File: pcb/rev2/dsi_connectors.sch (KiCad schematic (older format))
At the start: 6 parts, among them CN2 AX3E41264, CN3 CONN_02X15_ALT

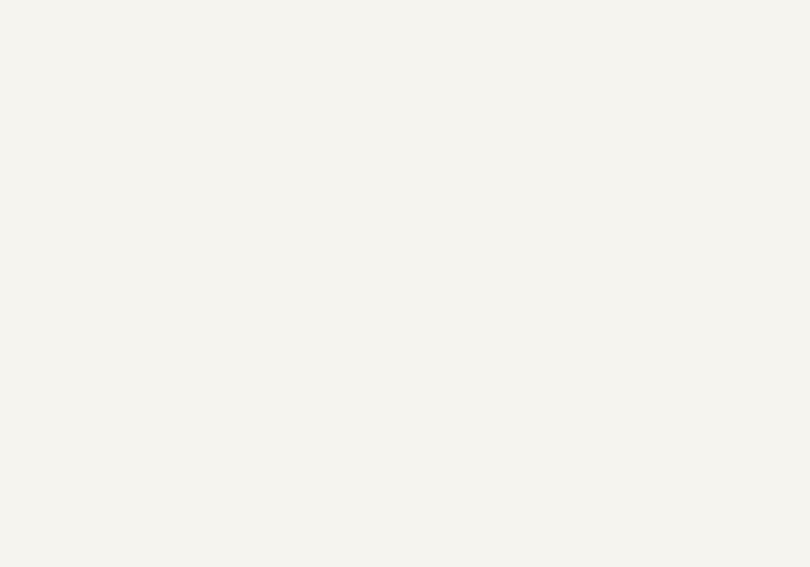
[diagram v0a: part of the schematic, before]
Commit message: pcb wip
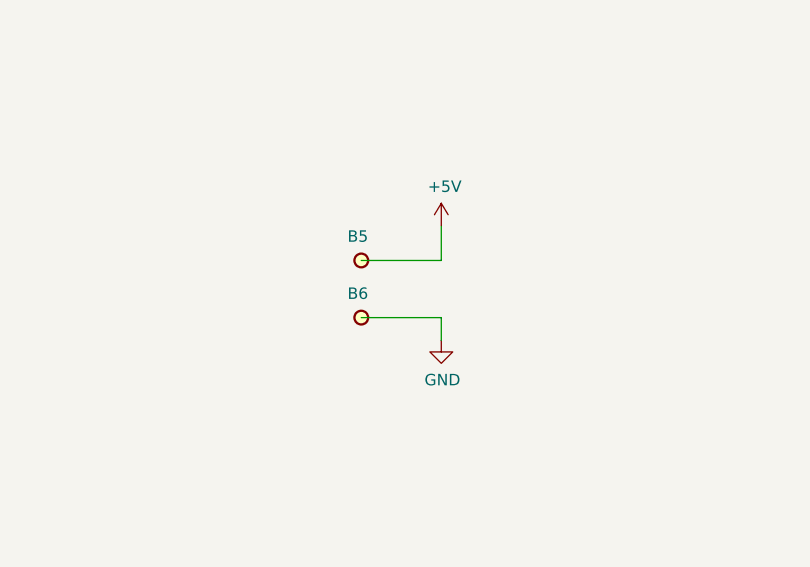
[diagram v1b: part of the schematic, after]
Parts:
- added B5, B6: PLATED_HOLE0.8_PAD1.3, c130h80, symbol PLATED_HOLE0.8_PAD1.3
- CN2: footprint (none) -> dsi_shield:IPHONE4_LCD_CONN
- CN3: footprint (none) -> dsi_shield:GB042-30S-E1000
- R1, R2, R49, R50: footprint RESC1608X55N -> Resistors SMD:RESC1608X55N
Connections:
- net labels added: +5V
- wire segments 79 -> 83
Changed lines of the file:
@@
 F 0 "CN2" H 6450 2865 50  0000 C CNN
 F 1 "AX3E41264" H 6450 2774 50  0000 C CNN
-F 2 "" H 6450 900 50  0001 C CNN
+F 2 "dsi_shield:IPHONE4_LCD_CONN" H 6450 900 50  0001 C CNN
 F 3 "" H 6450 900 50  0001 C CNN
 	1    6450 2050
@@
 F 0 "R1" H 7650 1853 50  0000 C CNN
 F 1 "R0603_10R_1%_0.1W_200PPM" H 7500 1340 60  0001 L CNN
-F 2 "RESC1608X55N" H 7500 530 60  0001 L CNN
+F 2 "Resistors SMD:RESC1608X55N" H 7500 530 60  0001 L CNN
 F 3 "\\cern.ch\\dfs\\Applications\\Altium\\Datasheets\\R0603_NIC_NRC.pdf" H 7500 1160 60  0001 L CNN
 F 4 "Value" H 7500 1550 60  0001 C CNN "Fieldname"
@@
 F 0 "R2" H 7650 2147 50  0000 C CNN
 F 1 "R0603_3K3_1%_0.1W_100PPM" H 7500 1740 60  0001 L CNN
-F 2 "RESC1608X55N" H 7500 930 60  0001 L CNN
+F 2 "Resistors SMD:RESC1608X55N" H 7500 930 60  0001 L CNN
 F 3 "\\cern.ch\\dfs\\Applications\\Altium\\Datasheets\\R0603_NIC_NRC.pdf" H 7500 1560 60  0001 L CNN
 F 4 "3k3" H 7650 2056 50  0000 C CNN "~"
@@
 F 0 "CN3" H 6450 5865 50  0000 C CNN
 F 1 "CONN_02X15_ALT" H 6450 5774 50  0000 C CNN
-F 2 "" H 6450 3800 50  0001 C CNN
+F 2 "dsi_shield:GB042-30S-E1000" H 6450 3800 50  0001 C CNN
 F 3 "" H 6450 3800 50  0001 C CNN
 	1    6450 4950
@@
 F 0 "R49" H 7300 4547 50  0000 C CNN
 F 1 "R0603_10R_1%_0.1W_200PPM" H 7150 4140 60  0001 L CNN
-F 2 "RESC1608X55N" H 7150 3330 60  0001 L CNN
+F 2 "Resistors SMD:RESC1608X55N" H 7150 3330 60  0001 L CNN
 F 3 "\\cern.ch\\dfs\\Applications\\Altium\\Datasheets\\R0603_NIC_NRC.pdf" H 7150 3960 60  0001 L CNN
 F 4 "10" H 7300 4456 50  0000 C CNN "~"
@@
 F 0 "R50" H 7300 4345 50  0000 C CNN
 F 1 "R0603_10R_1%_0.1W_200PPM" H 7150 4240 60  0001 L CNN
-F 2 "RESC1608X55N" H 7150 3430 60  0001 L CNN
+F 2 "Resistors SMD:RESC1608X55N" H 7150 3430 60  0001 L CNN
 F 3 "\\cern.ch\\dfs\\Applications\\Altium\\Datasheets\\R0603_NIC_NRC.pdf" H 7150 4060 60  0001 L CNN
 F 4 "10" H 7450 4350 50  0000 C CNN "~"
@@
 Wire Notes Line
 	3100 6800 700  6800
+$Comp
+L PLATED_HOLE0.8_PAD1.3 B5
+U 1 1 599E1A70
+P 2500 5000
+F 0 "B5" H 2485 5105 50  0000 C CNN
+F 1 "PLATED_HOLE0.8_PAD1.3" H 2500 4830 60  0001 L CNN
+F 2 "c130h80" H 2500 4020 60  0001 L CNN
+F 3 "Undefined" H 2500 4650 60  0001 L CNN
+F 4 "Plated Hole" H 2500 4560 60  0001 L CNN "Field4"
+F 5 "PLATED_HOLE0.8_PAD1.3" H 2500 4560 60  0001 L CNN "Part Number"
+F 6 "Single Terminal Socket" H 2500 4470 60  0001 L CNN "Library Ref"
+F 7 "SchLib\\Pads.SchLib" H 2500 4380 60  0001 L CNN "Library Path"
+F 8 "~~" H 2500 4290 60  0001 L CNN "Comment"
+F 9 "Standard (No BOM)" H 2500 4200 60  0001 L CNN "Component Kind"
+F 10 "Standard (No BOM)" H 2500 4110 60  0001 L CNN "Component Type"
+F 11 "1" H 2500 3930 60  0001 L CNN "Pin Count"
+F 12 "~~" H 2500 3840 60  0001 L CNN "Case"
+F 13 "PcbLib\\Pads.PcbLib" H 2500 3750 60  0001 L CNN "Footprint Path"
+F 14 "c130h80" H 2500 3660 60  0001 L CNN "Footprint Ref"
+F 15 "Plated Hole" H 2500 3570 60  0001 L CNN "Family"
+F 16 "No" H 2500 3480 60  0001 L CNN "Mounted"
+F 17 "No" H 2500 3390 60  0001 L CNN "Socket"
+F 18 "No" H 2500 3300 60  0001 L CNN "SMD"
+F 19 "No" H 2500 3210 60  0001 L CNN "Sense"
+F 20 "~~" H 2500 3120 60  0001 L CNN "Sense Comment"
+F 21 "None" H 2500 3030 60  0001 L CNN "Status"
+F 22 "~~" H 2500 2940 60  0001 L CNN "Status Comment"
+F 23 "~~" H 2500 2850 60  0001 L CNN "SCEM"
+F 24 "Plated Through Hole: Hole Dia.=0.8mm Pad Dia.=1.3mm, IPC-7251 Level C" H 2500 2760 60  0001 L CNN "Part Description"
+F 25 "~~" H 2500 2670 60  0001 L CNN "Manufacturer"
+F 26 "~~" H 2500 2580 60  0001 L CNN "Manufacturer Part Number"
+F 27 "0mm" H 2500 2490 60  0001 L CNN "ComponentHeight"
+F 28 "~~" H 2500 2400 60  0001 L CNN "Manufacturer1 Example"
+F 29 "~~" H 2500 2310 60  0001 L CNN "Manufacturer1 Part Number"
+F 30 "~~" H 2500 2220 60  0001 L CNN "Manufacturer1 ComponentHeight"
+F 31 "Undefined" H 2500 2130 60  0001 L CNN "HelpURL"
+F 32 "~~" H 2500 2040 60  0001 L CNN "ComponentLink1URL"
+F 33 "~~" H 2500 1950 60  0001 L CNN "ComponentLink1Description"
+F 34 "~~" H 2500 1860 60  0001 L CNN "ComponentLink2URL"
+F 35 "~~" H 2500 1770 60  0001 L CNN "ComponentLink2Description"
+F 36 "CERN DEM JLC" H 2500 1680 60  0001 L CNN "Author"
+F 37 "10/30/08 00:00:00" H 2500 1590 60  0001 L CNN "CreateDate"
+F 38 "10/30/08 00:00:00" H 2500 1500 60  0001 L CNN "LatestRevisionDate"
+F 39 "Plated Through Hole: Hole Dia.=0.8mm Pad Dia.=1.3mm, IPC-7251 Level C" H 2500 1410 60  0001 L CNN "PackageDescription"
+F 40 "Pads" H 2500 1320 60  0001 L CNN "Library Name"
+F 41 "This work is licensed under the Creative Commons CC-BY-SA 4.0 License. To the extent that circuit schematics that use Licensed Material can be considered to be ‘Adapted Material’, then the copyright holder waives article 3.b of the license with respect to these schematics." H 2500 1230 60  0001 L CNN "License"
+	1    2500 5000
+	1    0    0    -1
+$EndComp
+$Comp
+L PLATED_HOLE0.8_PAD1.3 B6
+U 1 1 599E1C02
+P 2500 5250
+F 0 "B6" H 2485 5355 50  0000 C CNN
+F 1 "PLATED_HOLE0.8_PAD1.3" H 2500 5080 60  0001 L CNN
+F 2 "c130h80" H 2500 4270 60  0001 L CNN
+F 3 "Undefined" H 2500 4900 60  0001 L CNN
+F 4 "Plated Hole" H 2500 4810 60  0001 L CNN "Field4"
+F 5 "PLATED_HOLE0.8_PAD1.3" H 2500 4810 60  0001 L CNN "Part Number"
+F 6 "Single Terminal Socket" H 2500 4720 60  0001 L CNN "Library Ref"
+F 7 "SchLib\\Pads.SchLib" H 2500 4630 60  0001 L CNN "Library Path"
+F 8 "~~" H 2500 4540 60  0001 L CNN "Comment"
+F 9 "Standard (No BOM)" H 2500 4450 60  0001 L CNN "Component Kind"
+F 10 "Standard (No BOM)" H 2500 4360 60  0001 L CNN "Component Type"
+F 11 "1" H 2500 4180 60  0001 L CNN "Pin Count"
+F 12 "~~" H 2500 4090 60  0001 L CNN "Case"
+F 13 "PcbLib\\Pads.PcbLib" H 2500 4000 60  0001 L CNN "Footprint Path"
+F 14 "c130h80" H 2500 3910 60  0001 L CNN "Footprint Ref"
+F 15 "Plated Hole" H 2500 3820 60  0001 L CNN "Family"
+F 16 "No" H 2500 3730 60  0001 L CNN "Mounted"
+F 17 "No" H 2500 3640 60  0001 L CNN "Socket"
+F 18 "No" H 2500 3550 60  0001 L CNN "SMD"
+F 19 "No" H 2500 3460 60  0001 L CNN "Sense"
+F 20 "~~" H 2500 3370 60  0001 L CNN "Sense Comment"
+F 21 "None" H 2500 3280 60  0001 L CNN "Status"
+F 22 "~~" H 2500 3190 60  0001 L CNN "Status Comment"
+F 23 "~~" H 2500 3100 60  0001 L CNN "SCEM"
+F 24 "Plated Through Hole: Hole Dia.=0.8mm Pad Dia.=1.3mm, IPC-7251 Level C" H 2500 3010 60  0001 L CNN "Part Description"
+F 25 "~~" H 2500 2920 60  0001 L CNN "Manufacturer"
+F 26 "~~" H 2500 2830 60  0001 L CNN "Manufacturer Part Number"
+F 27 "0mm" H 2500 2740 60  0001 L CNN "ComponentHeight"
+F 28 "~~" H 2500 2650 60  0001 L CNN "Manufacturer1 Example"
+F 29 "~~" H 2500 2560 60  0001 L CNN "Manufacturer1 Part Number"
+F 30 "~~" H 2500 2470 60  0001 L CNN "Manufacturer1 ComponentHeight"
+F 31 "Undefined" H 2500 2380 60  0001 L CNN "HelpURL"
+F 32 "~~" H 2500 2290 60  0001 L CNN "ComponentLink1URL"
+F 33 "~~" H 2500 2200 60  0001 L CNN "ComponentLink1Description"
+F 34 "~~" H 2500 2110 60  0001 L CNN "ComponentLink2URL"
+F 35 "~~" H 2500 2020 60  0001 L CNN "ComponentLink2Description"
+F 36 "CERN DEM JLC" H 2500 1930 60  0001 L CNN "Author"
+F 37 "10/30/08 00:00:00" H 2500 1840 60  0001 L CNN "CreateDate"
+F 38 "10/30/08 00:00:00" H 2500 1750 60  0001 L CNN "LatestRevisionDate"
+F 39 "Plated Through Hole: Hole Dia.=0.8mm Pad Dia.=1.3mm, IPC-7251 Level C" H 2500 1660 60  0001 L CNN "PackageDescription"
+F 40 "Pads" H 2500 1570 60  0001 L CNN "Library Name"
+F 41 "This work is licensed under the Creative Commons CC-BY-SA 4.0 License. To the extent that circuit schematics that use Licensed Material can be considered to be ‘Adapted Material’, then the copyright holder waives article 3.b of the license with respect to these schematics." H 2500 1480 60  0001 L CNN "License"
+	1    2500 5250
+	1    0    0    -1
+$EndComp
+$Comp
+L GND #PWR?
+U 1 1 599E1E7E
+P 2850 5350
+F 0 "#PWR?" H 2850 5100 50  0001 C CNN
+F 1 "GND" H 2855 5177 50  0000 C CNN
+F 2 "" H 2850 5350 50  0001 C CNN
+F 3 "" H 2850 5350 50  0001 C CNN
+	1    2850 5350
+	1    0    0    -1
+$EndComp
+Wire Wire Line
+	2500 5250 2850 5250
+Wire Wire Line
+	2850 5250 2850 5350
+$Comp
+L +5V #PWR?
+U 1 1 599E219E
+P 2850 4850
+F 0 "#PWR?" H 2850 4700 50  0001 C CNN
+F 1 "+5V" H 2865 5023 50  0000 C CNN
+F 2 "" H 2850 4850 50  0001 C CNN
+F 3 "" H 2850 4850 50  0001 C CNN
+	1    2850 4850
+	1    0    0    -1
+$EndComp
+Wire Wire Line
+	2500 5000 2850 5000
+Wire Wire Line
+	2850 5000 2850 4850
 $EndSCHEMATC
